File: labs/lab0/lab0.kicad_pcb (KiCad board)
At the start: 2 copper layers, 49.7 x 48.1 mm, 6 parts, among them J1 Conn_01x02_Pin, J2 Conn_01x02_Pin

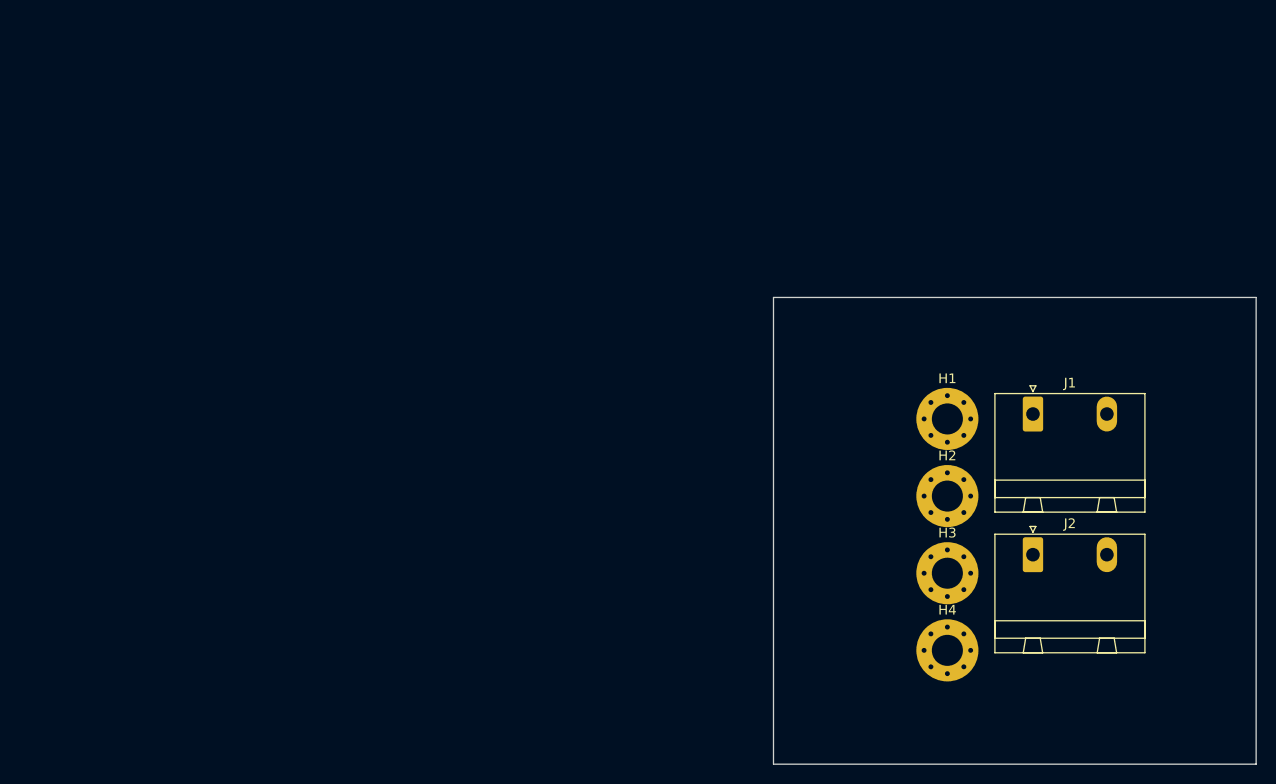
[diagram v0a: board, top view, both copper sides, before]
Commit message: lab0 finished
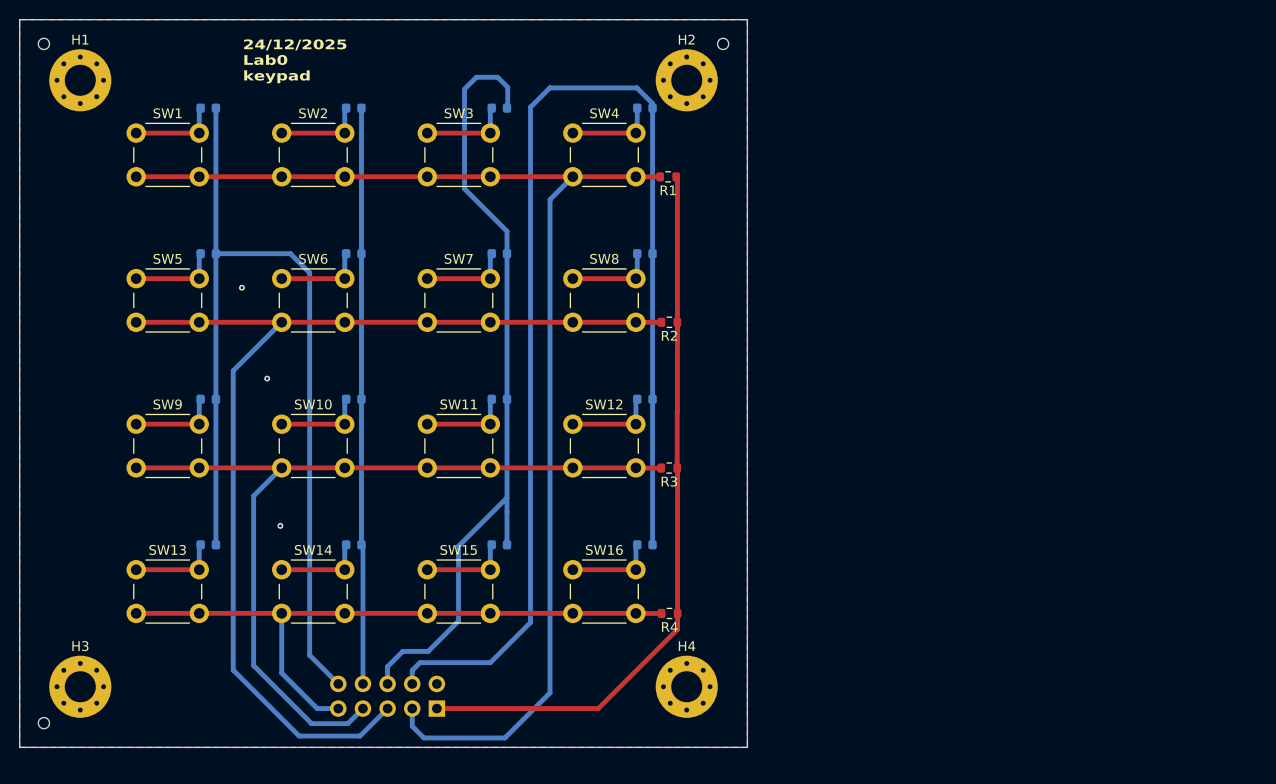
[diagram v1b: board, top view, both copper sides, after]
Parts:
- removed J2: Conn_01x02_Pin, Connector_Phoenix_GMSTB:PhoenixContact_GMSTBA_2,5_2-G-7,62_1x02_P7.62mm_Horizontal
- added D1: D, Diode_SMD:D_0603_1608Metric, B.Cu at (44.4, 34.1)
- added D10: D, Diode_SMD:D_0603_1608Metric, B.Cu at (59.4, 64.1)
- added D11: D, Diode_SMD:D_0603_1608Metric, B.Cu at (74.4, 64.1)
- added D12: D, Diode_SMD:D_0603_1608Metric, B.Cu at (89.4, 64.1)
- added D13: D, Diode_SMD:D_0603_1608Metric, B.Cu at (44.4, 79.1)
- added D14: D, Diode_SMD:D_0603_1608Metric, B.Cu at (59.4, 79.1)
- added D15: D, Diode_SMD:D_0603_1608Metric, B.Cu at (74.4, 79.1)
- added D16: D, Diode_SMD:D_0603_1608Metric, B.Cu at (89.4, 79.1)
- added D2: D, Diode_SMD:D_0603_1608Metric, B.Cu at (59.4, 34.1)
- added D3: D, Diode_SMD:D_0603_1608Metric, B.Cu at (74.4, 34.1)
- added D4: D, Diode_SMD:D_0603_1608Metric, B.Cu at (89.4, 34.1)
- added D5: D, Diode_SMD:D_0603_1608Metric, B.Cu at (44.4, 49.1)
- added D6: D, Diode_SMD:D_0603_1608Metric, B.Cu at (59.4, 49.1)
- added D7: D, Diode_SMD:D_0603_1608Metric, B.Cu at (74.4, 49.1)
- added D8: D, Diode_SMD:D_0603_1608Metric, B.Cu at (89.4, 49.1)
- added D9: D, Diode_SMD:D_0603_1608Metric, B.Cu at (44.4, 64.1)
- added H5: MountingHole, MountingHole:ToolingHole_1.152mm, F.Cu at (27.5, 27.5)
- added H6: MountingHole, MountingHole:ToolingHole_1.152mm, F.Cu at (97.5, 27.5)
- added H7: MountingHole, MountingHole:ToolingHole_1.152mm, F.Cu at (27.5, 97.5)
- added R1: 10k, Resistor_SMD:R_0603_1608Metric, F.Cu at (91.8, 41.2)
- added R2: 10k, Resistor_SMD:R_0603_1608Metric, F.Cu at (92.0, 56.2)
- added R3: 10k, Resistor_SMD:R_0603_1608Metric, F.Cu at (91.9, 71.2)
- added R4: 10k, Resistor_SMD:R_0603_1608Metric, F.Cu at (92.0, 86.2)
- added SW1: SW_Omron_B3FS, Button_Switch_THT:SW_PUSH_6mm, F.Cu at (37.0, 36.7)
- added SW10: SW_Omron_B3FS, Button_Switch_THT:SW_PUSH_6mm, F.Cu at (52.0, 66.7)
- added SW11: SW_Omron_B3FS, Button_Switch_THT:SW_PUSH_6mm, F.Cu at (67.0, 66.7)
- added SW12: SW_Omron_B3FS, Button_Switch_THT:SW_PUSH_6mm, F.Cu at (82.0, 66.7)
- added SW13: SW_Omron_B3FS, Button_Switch_THT:SW_PUSH_6mm, F.Cu at (37.0, 81.7)
- added SW14: SW_Omron_B3FS, Button_Switch_THT:SW_PUSH_6mm, F.Cu at (52.0, 81.7)
- added SW15: SW_Omron_B3FS, Button_Switch_THT:SW_PUSH_6mm, F.Cu at (67.0, 81.7)
- added SW16: SW_Omron_B3FS, Button_Switch_THT:SW_PUSH_6mm, F.Cu at (82.0, 81.7)
- added SW2: SW_Omron_B3FS, Button_Switch_THT:SW_PUSH_6mm, F.Cu at (52.0, 36.7)
- added SW3: SW_Omron_B3FS, Button_Switch_THT:SW_PUSH_6mm, F.Cu at (67.0, 36.7)
- added SW4: SW_Omron_B3FS, Button_Switch_THT:SW_PUSH_6mm, F.Cu at (82.0, 36.7)
- added SW5: SW_Omron_B3FS, Button_Switch_THT:SW_PUSH_6mm, F.Cu at (37.0, 51.7)
- added SW6: SW_Omron_B3FS, Button_Switch_THT:SW_PUSH_6mm, F.Cu at (52.0, 51.7)
- added SW7: SW_Omron_B3FS, Button_Switch_THT:SW_PUSH_6mm, F.Cu at (67.0, 51.7)
- added SW8: SW_Omron_B3FS, Button_Switch_THT:SW_PUSH_6mm, F.Cu at (82.0, 51.7)
- added SW9: SW_Omron_B3FS, Button_Switch_THT:SW_PUSH_6mm, F.Cu at (37.0, 66.7)
- J1: value Conn_01x02_Pin -> Conn_02x05_Odd_Even; footprint Connector_Phoenix_GMSTB:PhoenixContact_GMSTBA_2,5_2-G-7,62_1x02_P7.62mm_Horizontal -> Connector_PinHeader_2.54mm:PinHeader_2x05_P2.54mm_Vertical; moved to B.Cu
- moved H1 95.9 mm to (31.2, 31.2)
- moved H3 90.1 mm to (31.2, 93.8)
- moved J1 68.5 mm to (68.0, 96.0), turned to 90 degrees
- moved H2 50.6 mm to (93.8, 31.2)
- moved H4 27.1 mm to (93.8, 93.8)
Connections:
- J1 pad 1: unconnected-(J1-Pin_1-Pad1) -> VCC
- J1 pad 2: unconnected-(J1-Pin_2-Pad2) -> GND
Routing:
- net RAW_4: track 0.00 -> 128.3 mm
- net COL_1: track 0.00 -> 126.6 mm
- net COL_2: track 0.00 -> 111.9 mm
- net RAW_1: track 0.00 -> 99.1 mm
- net COL_3: track 0.00 -> 90.1 mm
- net RAW_3: track 0.00 -> 82.1 mm
- net VCC: track 0.00 -> 74.9 mm
- net COL_4: track 0.00 -> 67.6 mm
- net RAW_2: track 0.00 -> 59.4 mm
- net Net-(D6-A): track 0.00 -> 9.13 mm
- net Net-(D5-A): track 0.00 -> 9.13 mm
- net Net-(D2-A): track 0.00 -> 9.13 mm
- net Net-(D1-A): track 0.00 -> 9.13 mm
- net Net-(D8-A): track 0.00 -> 9.13 mm
- net Net-(D4-A): track 0.00 -> 9.13 mm
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- added copper zone on B.Cu, net GND
- added copper zone on F.Cu, net GND
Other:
- board size 49.7 x 48.1 mm -> 75 x 75 mm
- board text added: "24/12/2025 Lab0 keypad"
